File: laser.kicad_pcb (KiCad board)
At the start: 2 copper layers, 50 x 50 mm, 18 parts, among them J1 Conn_Coaxial, J2 Conn_02x06, J3 Conn_Coaxial, Q1 BS170, Q2 BS170

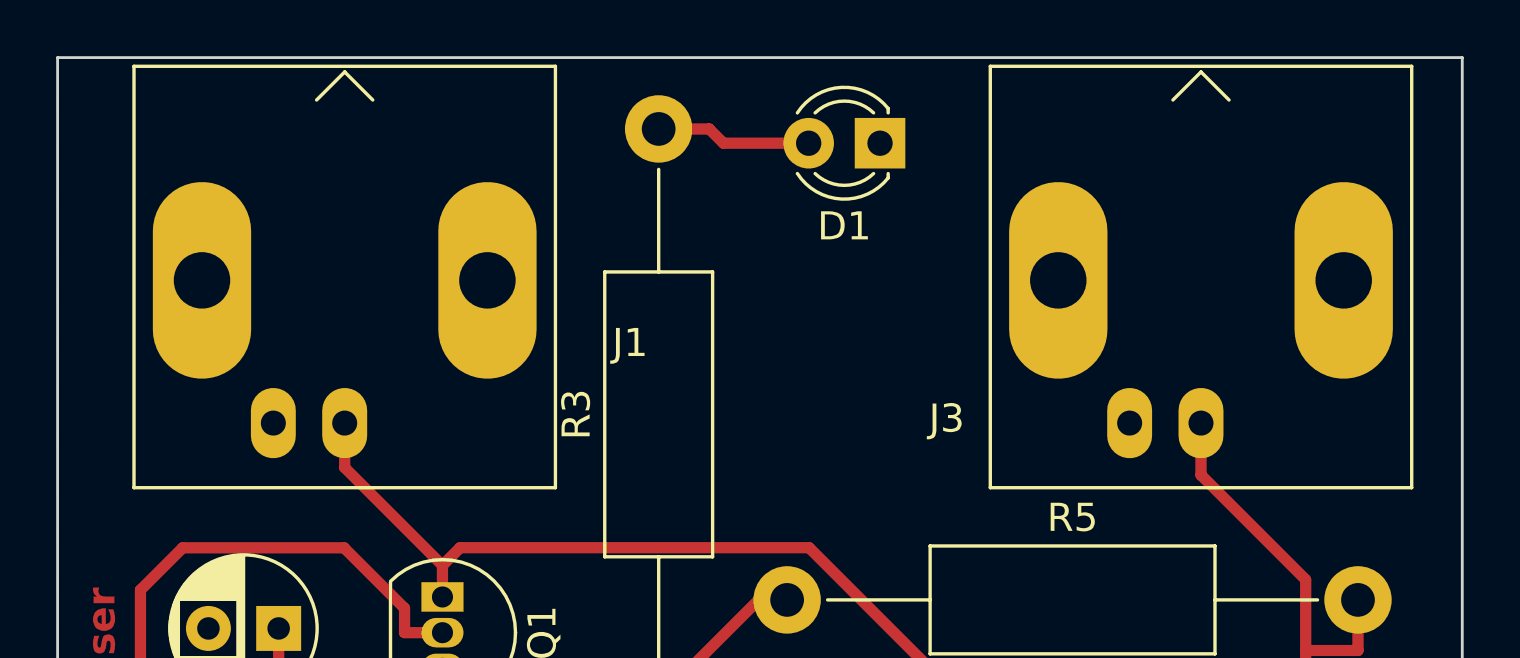
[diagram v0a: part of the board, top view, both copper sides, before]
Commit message: change the bnc connector of the backplane
change the bnc connector of the backplane
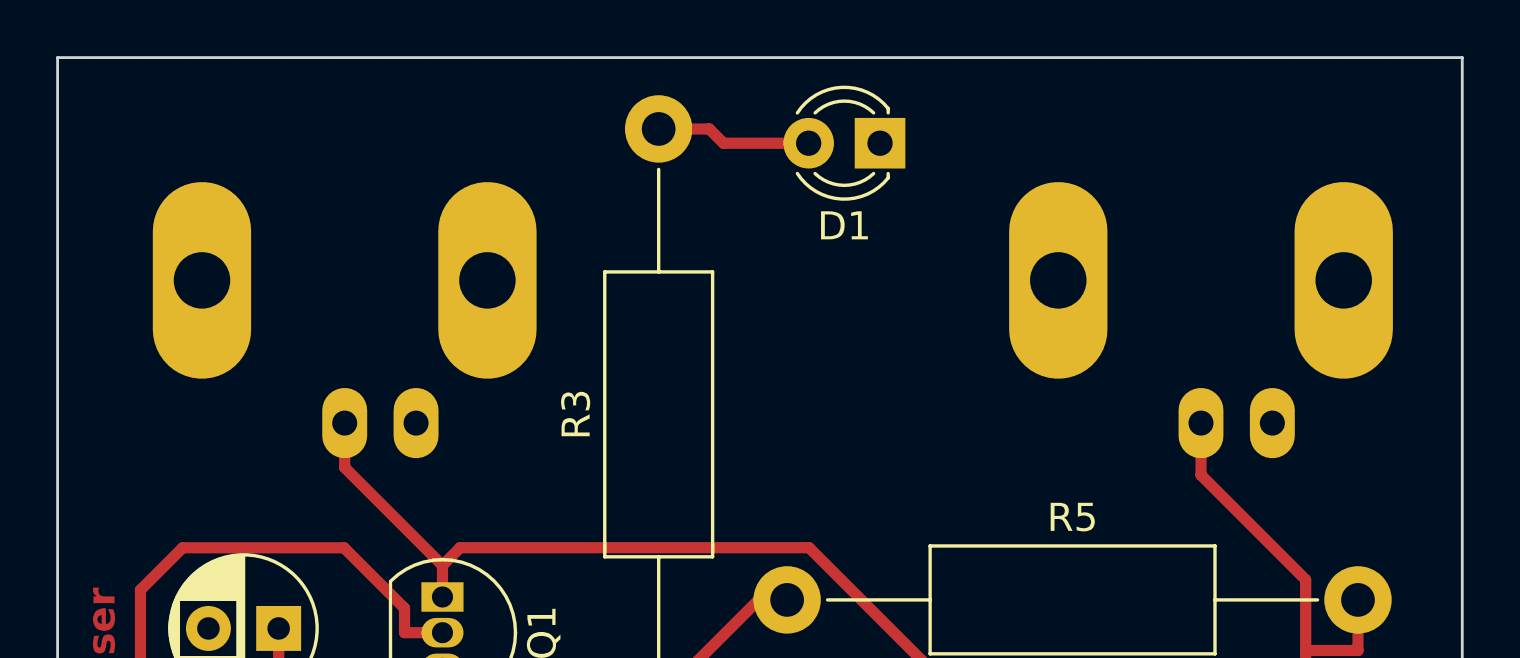
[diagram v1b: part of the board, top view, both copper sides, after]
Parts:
- J1, J3: moved to B.Cu
- turned J1 to 180 degrees
- turned J3 to 180 degrees
